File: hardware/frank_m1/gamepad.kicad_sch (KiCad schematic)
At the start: 3 parts, among them J7 D-SUB 9 Male

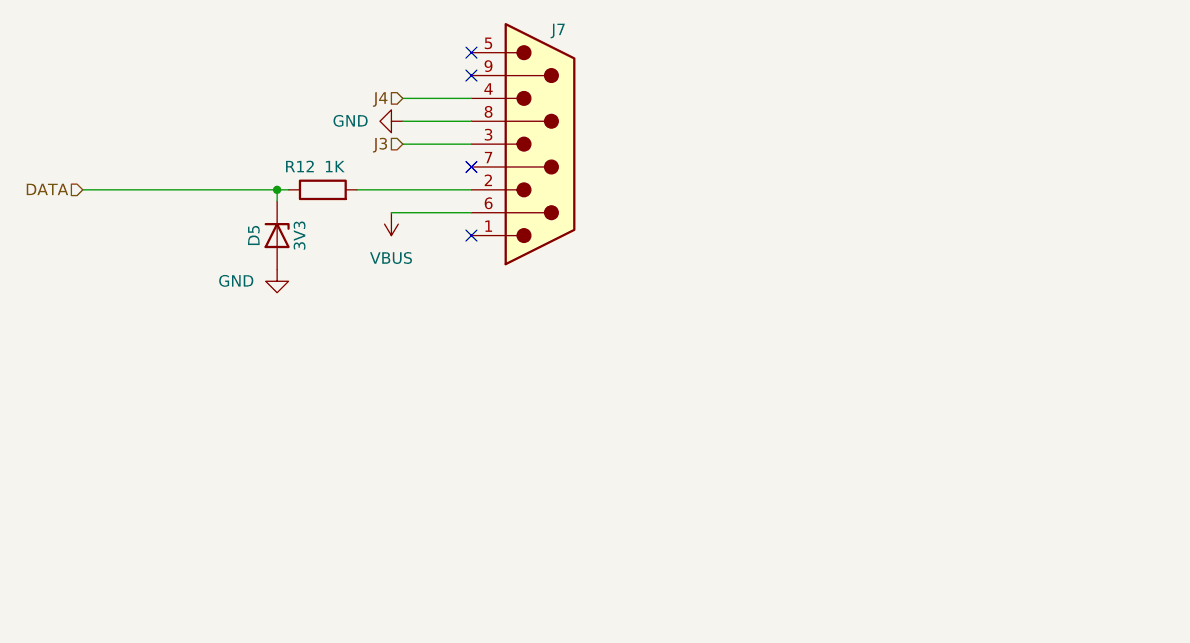
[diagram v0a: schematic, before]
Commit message: Minor updates
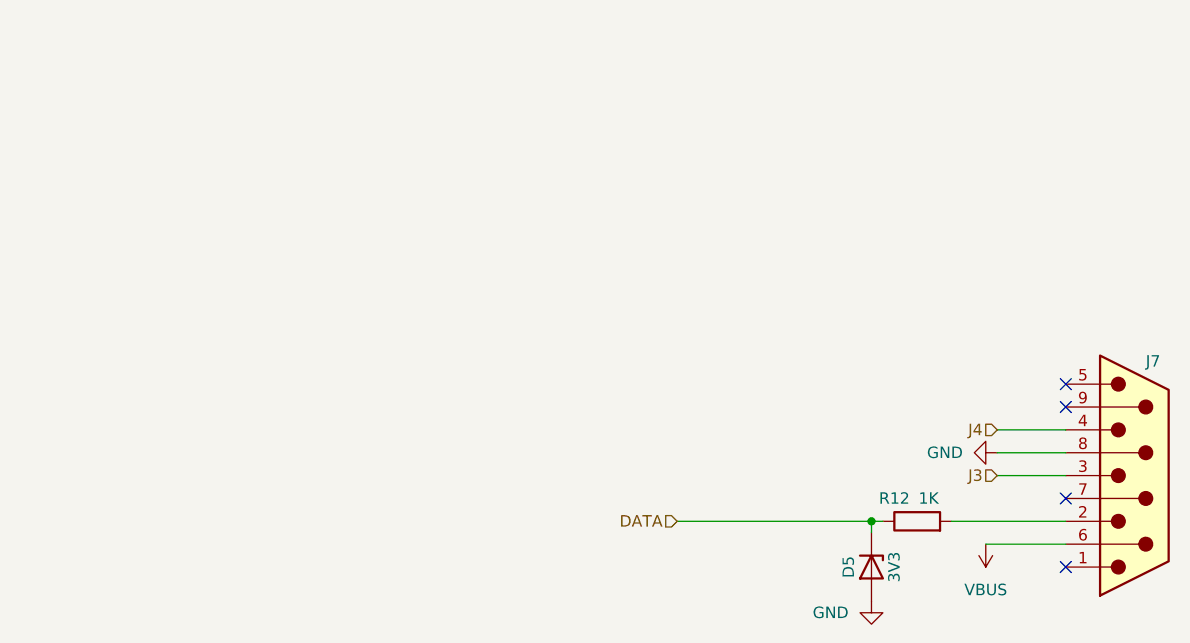
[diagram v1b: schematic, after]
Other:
- moved on the sheet: D5, J7, R12
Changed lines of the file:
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@@
 	)
 	(junction
-		(at 78.74 68.58)
+		(at 144.78 105.41)
 		(diameter 0)
 		(color 0 0 0 0)
 	)
 	(no_connect
-		(at 100.33 55.88)
+		(at 166.37 92.71)
 	)
 	(no_connect
-		(at 100.33 53.34)
+		(at 166.37 90.17)
 	)
 	(no_connect
-		(at 100.33 66.04)
+		(at 166.37 102.87)
 	)
 	(no_connect
-		(at 100.33 73.66)
-	)
-	(wire
-		(pts
-			(xy 92.71 63.5) (xy 100.33 63.5)
-		)
-		(stroke
-			(width 0)
-			(type default)
-		)
-	)
-	(wire
-		(pts
-			(xy 92.71 58.42) (xy 100.33 58.42)
-		)
-		(stroke
-			(width 0)
-			(type default)
-		)
-	)
-	(wire
-		(pts
-			(xy 91.44 71.12) (xy 100.33 71.12)
-		)
-		(stroke
-			(width 0)
-			(type default)
-		)
-	)
-	(wire
-		(pts
-			(xy 78.74 68.58) (xy 78.74 69.85)
-		)
-		(stroke
-			(width 0)
-			(type default)
-		)
-	)
-	(wire
-		(pts
-			(xy 57.15 68.58) (xy 78.74 68.58)
-		)
-		(stroke
-			(width 0)
-			(type default)
-		)
-	)
-	(wire
-		(pts
-			(xy 80.01 68.58) (xy 78.74 68.58)
-		)
-		(stroke
-			(width 0)
-			(type default)
-		)
-	)
-	(wire
-		(pts
-			(xy 92.71 60.96) (xy 100.33 60.96)
-		)
-		(stroke
-			(width 0)
-			(type default)
-		)
-	)
-	(wire
-		(pts
-			(xy 87.63 68.58) (xy 100.33 68.58)
+		(at 166.37 110.49)
+	)
+	(wire
+		(pts
+			(xy 158.75 100.33) (xy 166.37 100.33)
+		)
+		(stroke
+			(width 0)
+			(type default)
+		)
+	)
+	(wire
+		(pts
+			(xy 158.75 95.25) (xy 166.37 95.25)
+		)
+		(stroke
+			(width 0)
+			(type default)
+		)
+	)
+	(wire
+		(pts
+			(xy 157.48 107.95) (xy 166.37 107.95)
+		)
+		(stroke
+			(width 0)
+			(type default)
+		)
+	)
+	(wire
+		(pts
+			(xy 144.78 105.41) (xy 144.78 106.68)
+		)
+		(stroke
+			(width 0)
+			(type default)
+		)
+	)
+	(wire
+		(pts
+			(xy 123.19 105.41) (xy 144.78 105.41)
+		)
+		(stroke
+			(width 0)
+			(type default)
+		)
+	)
+	(wire
+		(pts
+			(xy 146.05 105.41) (xy 144.78 105.41)
+		)
+		(stroke
+			(width 0)
+			(type default)
+		)
+	)
+	(wire
+		(pts
+			(xy 158.75 97.79) (xy 166.37 97.79)
+		)
+		(stroke
+			(width 0)
+			(type default)
+		)
+	)
+	(wire
+		(pts
+			(xy 153.67 105.41) (xy 166.37 105.41)
 		)
 		(stroke
@@
 	(hierarchical_label "J4"
 		(shape input)
-		(at 92.71 58.42 180)
+		(at 158.75 95.25 180)
 		(effects
 			(font
@@
 	(hierarchical_label "J3"
 		(shape input)
-		(at 92.71 63.5 180)
+		(at 158.75 100.33 180)
 		(effects
 			(font
@@
 	(hierarchical_label "DATA"
 		(shape input)
-		(at 57.15 68.58 180)
+		(at 123.19 105.41 180)
 		(effects
 			(font
@@
 	(symbol
 		(lib_id "power:GND")
-		(at 78.74 77.47 0)
+		(at 144.78 114.3 0)
 		(unit 1)
 		(exclude_from_sim no)
@@
 		(dnp no)
 		(property "Reference" "#PWR034"
-			(at 78.74 83.82 0)
+			(at 144.78 120.65 0)
 			(effects
 				(font
@@
 		)
 		(property "Value" "GND"
-			(at 76.2 78.74 0)
+			(at 142.24 115.57 0)
 			(effects
 				(font
@@
 		)
 		(property "Footprint" ""
-			(at 78.74 77.47 0)
+			(at 144.78 114.3 0)
 			(effects
 				(font
@@
 		)
 		(property "Datasheet" ""
-			(at 78.74 77.47 0)
+			(at 144.78 114.3 0)
 			(effects
 				(font
@@
 		)
 		(property "Description" "Power symbol creates a global label with name \"GND\" , ground"
-			(at 78.74 77.47 0)
+			(at 144.78 114.3 0)
 			(effects
 				(font
@@
 	(symbol
 		(lib_id "Device:D_Zener")
-		(at 78.74 73.66 270)
+		(at 144.78 110.49 270)
 		(unit 1)
 		(exclude_from_sim no)
@@
 		(dnp no)
 		(property "Reference" "D5"
-			(at 76.2 73.66 0)
+			(at 142.24 110.49 0)
 			(effects
 				(font
@@
 		)
 		(property "Value" "3V3"
-			(at 81.28 73.66 0)
+			(at 147.32 110.49 0)
 			(effects
 				(font
@@
 		)
 		(property "Footprint" "FRANK:Diode (SOD-323)"
-			(at 78.74 73.66 0)
+			(at 144.78 110.49 0)
 			(effects
 				(font
@@
 		)
 		(property "Datasheet" "https://www.vishay.com/docs/83335/bzx384g.pdf"
-			(at 78.74 73.66 0)
+			(at 144.78 110.49 0)
 			(effects
 				(font
@@
 		)
 		(property "Description" ""
-			(at 78.74 73.66 0)
+			(at 144.78 110.49 0)
 			(effects
 				(font
@@
 		)
 		(property "AliExpress" "https://www.aliexpress.com/item/1005006143480992.html"
-			(at 78.74 73.66 0)
+			(at 144.78 110.49 0)
 			(effects
 				(font
@@
 	(symbol
 		(lib_id "power:VBUS")
-		(at 91.44 71.12 180)
+		(at 157.48 107.95 180)
 		(unit 1)
 		(exclude_from_sim no)
@@
 		(fields_autoplaced yes)
 		(property "Reference" "#PWR033"
-			(at 91.44 67.31 0)
+			(at 157.48 104.14 0)
 			(effects
 				(font
@@
 		)
 		(property "Value" "VBUS"
-			(at 91.44 76.2 0)
+			(at 157.48 113.03 0)
 			(effects
 				(font
@@
 		)
 		(property "Footprint" ""
-			(at 91.44 71.12 0)
+			(at 157.48 107.95 0)
 			(effects
 				(font
@@
 		)
 		(property "Datasheet" ""
-			(at 91.44 71.12 0)
+			(at 157.48 107.95 0)
 			(effects
 				(font
@@
 		)
 		(property "Description" "Power symbol creates a global label with name \"VBUS\""
-			(at 91.44 71.12 0)
+			(at 157.48 107.95 0)
 			(effects
 				(font
@@
 	(symbol
 		(lib_id "FRANK:DB9_Male_Small")
-		(at 107.95 63.5 0)
+		(at 173.99 100.33 0)
 		(unit 1)
 		(exclude_from_sim no)
@@
 		(dnp no)
 		(property "Reference" "J7"
-			(at 109.22 50.8 0)
+			(at 175.26 87.63 0)
 			(effects
 				(font
@@
 		)
 		(property "Value" "D-SUB 9 Male"
-			(at 105.41 48.26 0)
+			(at 171.45 85.09 0)
 			(effects
 				(font
@@
 		)
 		(property "Footprint" "FRANK:D-SUB (9 pin, male, top mount)"
-			(at 107.95 63.5 0)
+			(at 173.99 100.33 0)
 			(effects
 				(font
@@
 		)
 		(property "Datasheet" "https://eu.mouser.com/datasheet/2/578/original-3313093.pdf"
-			(at 107.95 63.5 0)
+			(at 173.99 100.33 0)
 			(effects
 				(font
@@
 		)
 		(property "Description" ""
-			(at 107.95 63.5 0)
+			(at 173.99 100.33 0)
 			(effects
 				(font
@@
 		)
 		(property "AliExpress" "https://www.aliexpress.com/item/4001214300548.html"
-			(at 107.95 63.5 0)
+			(at 173.99 100.33 0)
 			(effects
 				(font
@@
 		(lib_name "GND_1")
 		(lib_id "power:GND")
-		(at 92.71 60.96 270)
+		(at 158.75 97.79 270)
 		(unit 1)
 		(exclude_from_sim no)
@@
 		(fields_autoplaced yes)
 		(property "Reference" "#PWR032"
-			(at 86.36 60.96 0)
+			(at 152.4 97.79 0)
 			(effects
 				(font
@@
 		)
 		(property "Value" "GND"
-			(at 88.9 60.9599 90)
+			(at 154.94 97.7899 90)
 			(effects
 				(font
@@
 		)
 		(property "Footprint" ""
-			(at 92.71 60.96 0)
+			(at 158.75 97.79 0)
 			(effects
 				(font
@@
 		)
 		(property "Datasheet" ""
-			(at 92.71 60.96 0)
+			(at 158.75 97.79 0)
 			(effects
 				(font
@@
 		)
 		(property "Description" "Power symbol creates a global label with name \"GND\" , ground"
-			(at 92.71 60.96 0)
+			(at 158.75 97.79 0)
 			(effects
 				(font
@@
 	(symbol
 		(lib_id "Device:R")
-		(at 83.82 68.58 90)
+		(at 149.86 105.41 90)
 		(unit 1)
 		(exclude_from_sim no)
@@
 		(dnp no)
 		(property "Reference" "R12"
-			(at 81.28 66.04 90)
+			(at 147.32 102.87 90)
 			(effects
 				(font
@@
 		)
 		(property "Value" "1K"
-			(at 85.09 66.04 90)
+			(at 151.13 102.87 90)
 			(effects
 				(font
@@
 		)
 		(property "Footprint" "FRANK:Resistor (0805)"
-			(at 83.82 70.358 90)
+			(at 149.86 107.188 90)
 			(effects
 				(font
@@
 		)
 		(property "Datasheet" "https://www.vishay.com/docs/28952/mcs0402at-mct0603at-mcu0805at-mca1206at.pdf"
-			(at 83.82 68.58 0)
+			(at 149.86 105.41 0)
 			(effects
 				(font
@@
 		)
 		(property "Description" ""
-			(at 83.82 68.58 0)
+			(at 149.86 105.41 0)
 			(effects
 				(font
@@
 		)
 		(property "AliExpress" "https://www.aliexpress.com/item/1005005945735199.html"
-			(at 83.82 68.58 0)
-			(effects
-				(font
+			(at 149.86 105.41 0)
+			(effects
+				(font
